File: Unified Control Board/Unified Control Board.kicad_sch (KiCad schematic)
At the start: 167 parts, among them CN1 B02B-PASK(LF)(SN), CN10 B3B-XH-2(LF)(SN), CN11 B3B-XH-2(LF)(SN), CN2 B02B-PASK(LF)(SN), CN3 B02B-PASK(LF)(SN), CN4 B04B-PASK(LF)(SN), CN5 B04B-PASK(LF)(SN), CN6 B02B-PASK(LF)(SN), CN7 B04B-PASK(LF)(SN), CN8 B04B-PASK(LF)(SN), CN9 B3B-XH-2(LF)(SN), SW1 TSA002A3512A02, SW2 TSA002A3512A02, SW3 TSA002A3512A02, U1 XT60PB-M.G.Y, U10 2.4GHz, U11 MP6541A, U12 MP6541A, U2 DRV8876PWPR, U3 DRV8876PWPR, U4 DRV8876PWPR, U5 DRV8876PWPR, U6 TCA9546A, U7 ZDSD01GLGEAG, U8 ESP32-S3-WROOM-1, U9 AP64350SP-13

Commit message: Before thermal vias
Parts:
- removed USB2: TYPE-C 16PIN, ProPrj_Dri-easyedapro:USB-C-SMD_TYPE-C-6PIN-2MD-073, symbol ProPrj_Dri-easyedapro:TYPE-C 16PIN 2MD(073)
- added USB2: KH-TYPE-C-16P, MaslowMerged:USB-C-SMD_KH-TYPE-C-16P, symbol KH-TYPE-C-16P
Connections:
- net CC1: now also USB2.A5 (CC1)
- net CC2: now also USB2.B5 (CC2)
- net D+: now also USB2.A6 (DP1), USB2.B6 (DP2)
- net D-: now also USB2.A7 (DN1), USB2.B7 (DN2)
- net GND: now also USB2.1 (EP), USB2.2 (EP), USB2.3 (EP), USB2.4 (EP), USB2.A1 (GND), USB2.A12 (GND), USB2.B1 (GND), USB2.B12 (GND)
- net VBUS: now also USB2.A4 (VBUS), USB2.A9 (VBUS), USB2.B4 (VBUS), USB2.B9 (VBUS)
- no-connect marks 31 -> 29
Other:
- moved on the sheet: C1, C10, C11, C12, C13, C14, C15, C16, C17, C18, C19, C2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

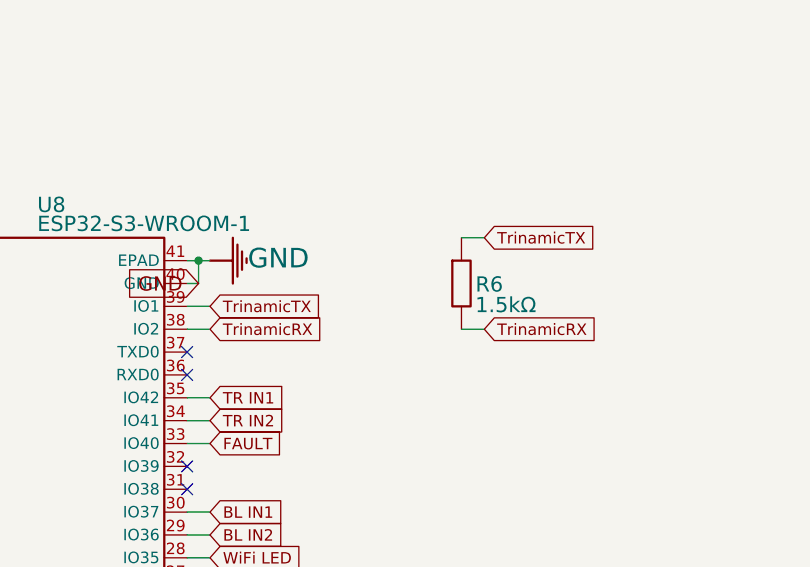
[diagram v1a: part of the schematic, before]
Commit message: Two wires left to route
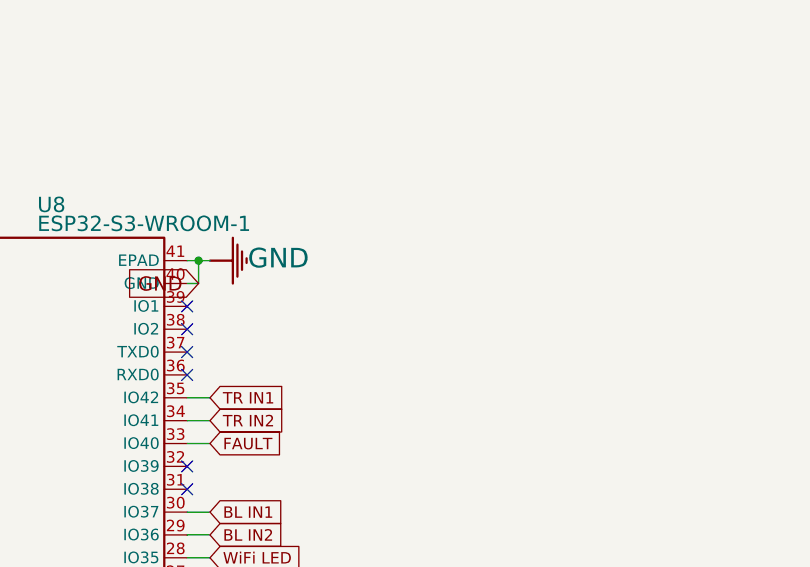
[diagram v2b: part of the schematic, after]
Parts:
- removed R6: 1.5kΩ, ProPrj_Dri-easyedapro:R0402, symbol 0805W8F1501T5E_4
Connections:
- net TrinamicRX: no longer names the net of U8.38 (IO2)
- net TrinamicTX: no longer names the net of U8.39 (IO1)
- no-connect marks 29 -> 31
